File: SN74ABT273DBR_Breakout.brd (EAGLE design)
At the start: 17.8 x 25.4 mm, 3 parts, among them IC1 SN74ABT273DBR

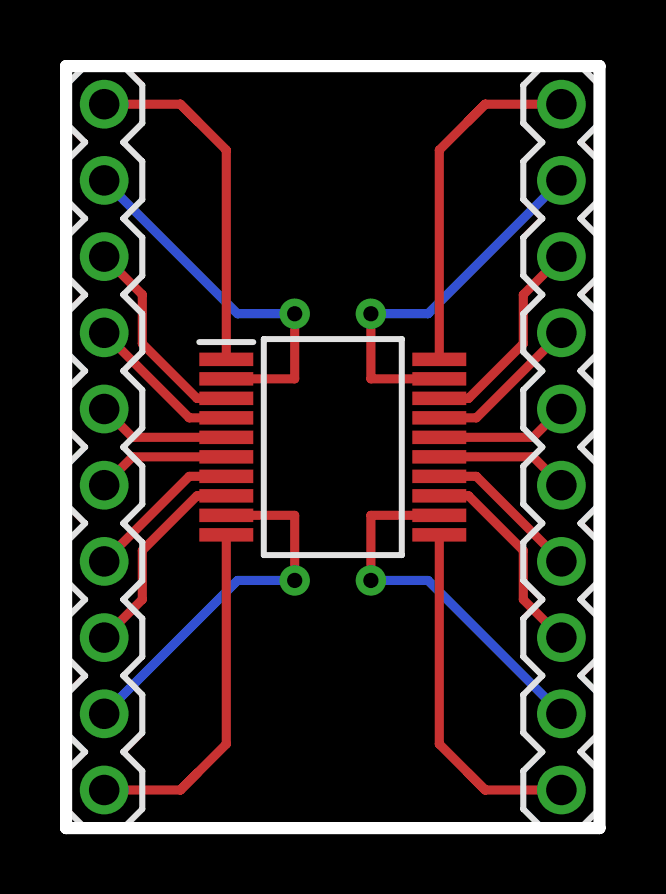
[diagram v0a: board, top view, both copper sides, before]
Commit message: Finished design and generated gerbers
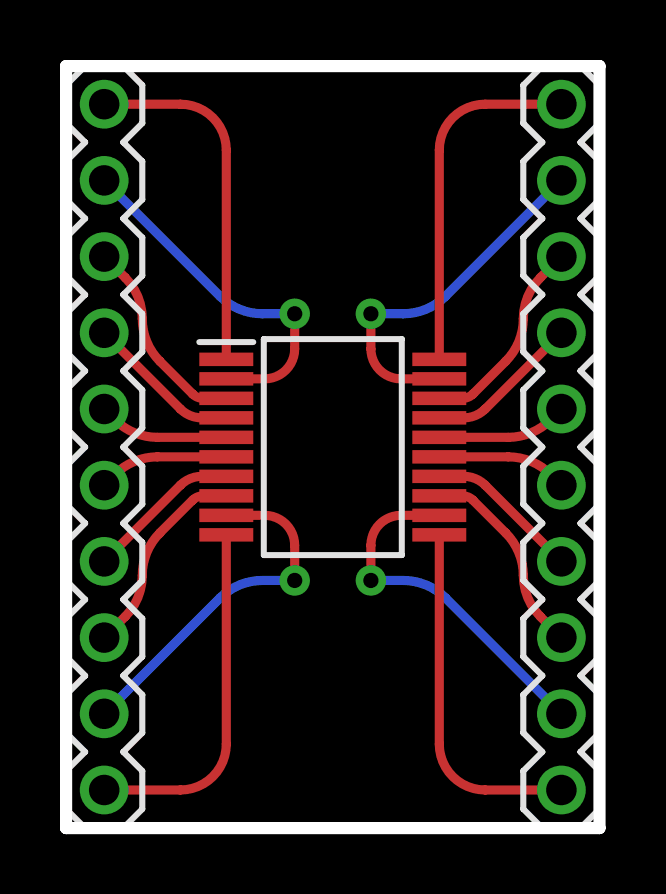
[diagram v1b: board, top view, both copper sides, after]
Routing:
- net N$20: track 12.5 -> 11.7 mm
- net N$1: track 12.5 -> 11.7 mm
- net N$11: track 12.5 -> 11.7 mm
- net N$10: track 12.5 -> 11.7 mm
- net N$9: track 12.6 -> 11.9 mm
- net N$2: track 12.6 -> 11.9 mm
- net N$12: track 12.6 -> 11.9 mm
- net N$19: track 12.6 -> 11.9 mm
